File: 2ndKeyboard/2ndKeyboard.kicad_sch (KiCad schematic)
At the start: 21 parts

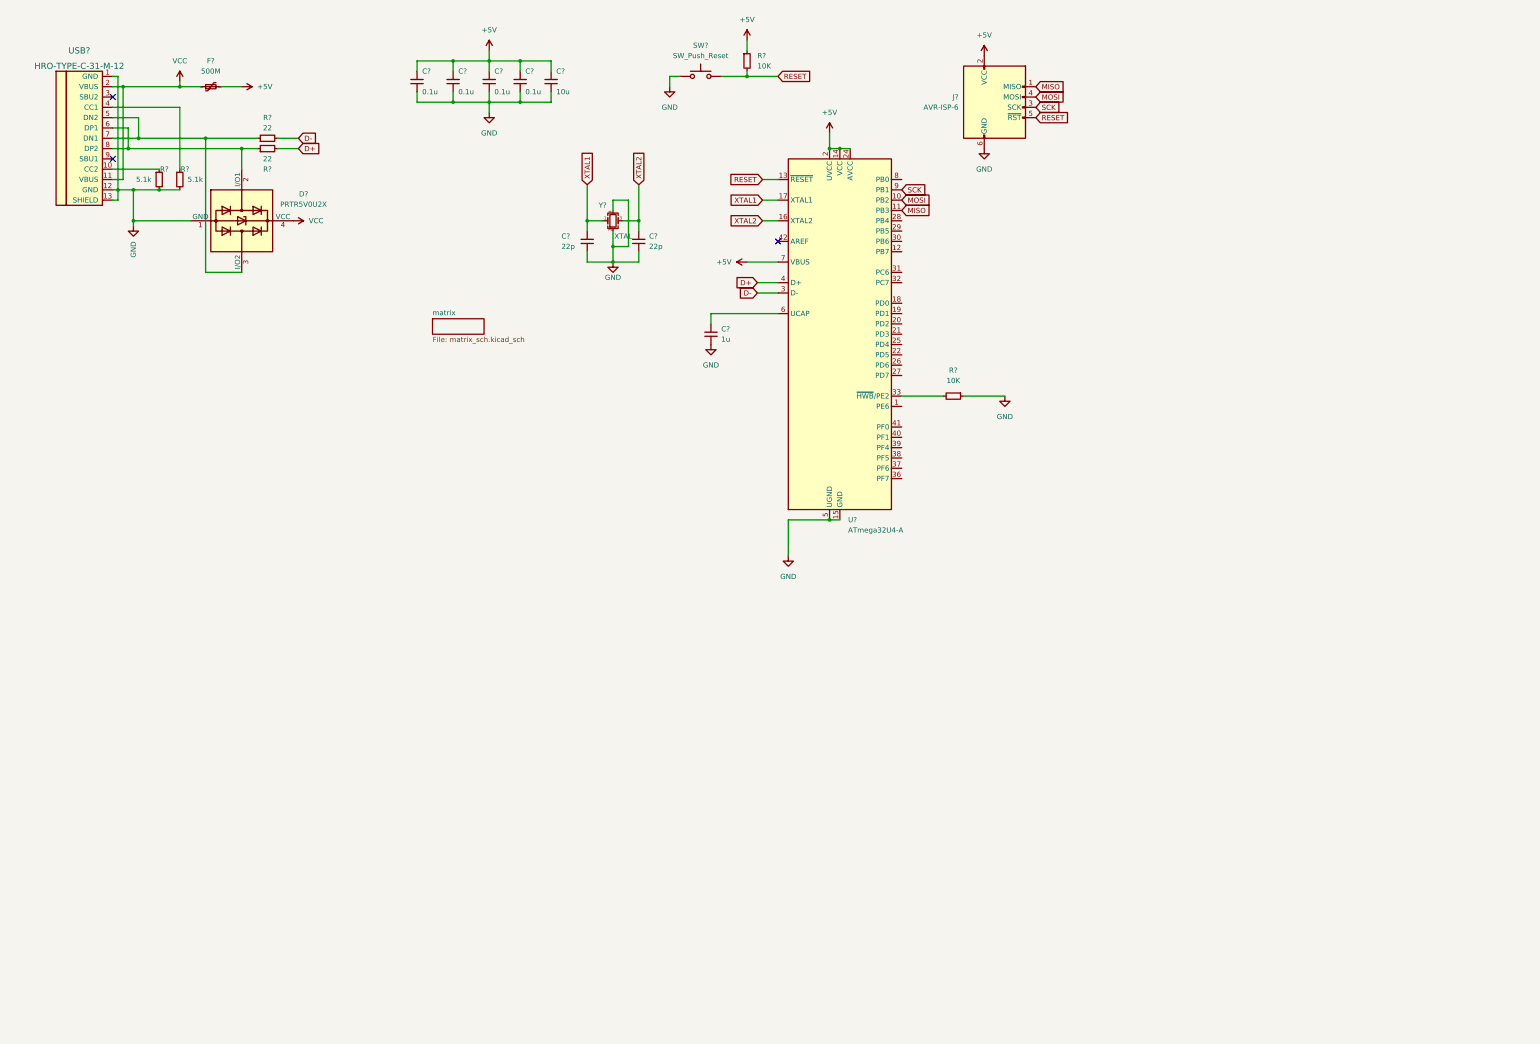
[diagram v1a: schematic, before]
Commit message: pcb
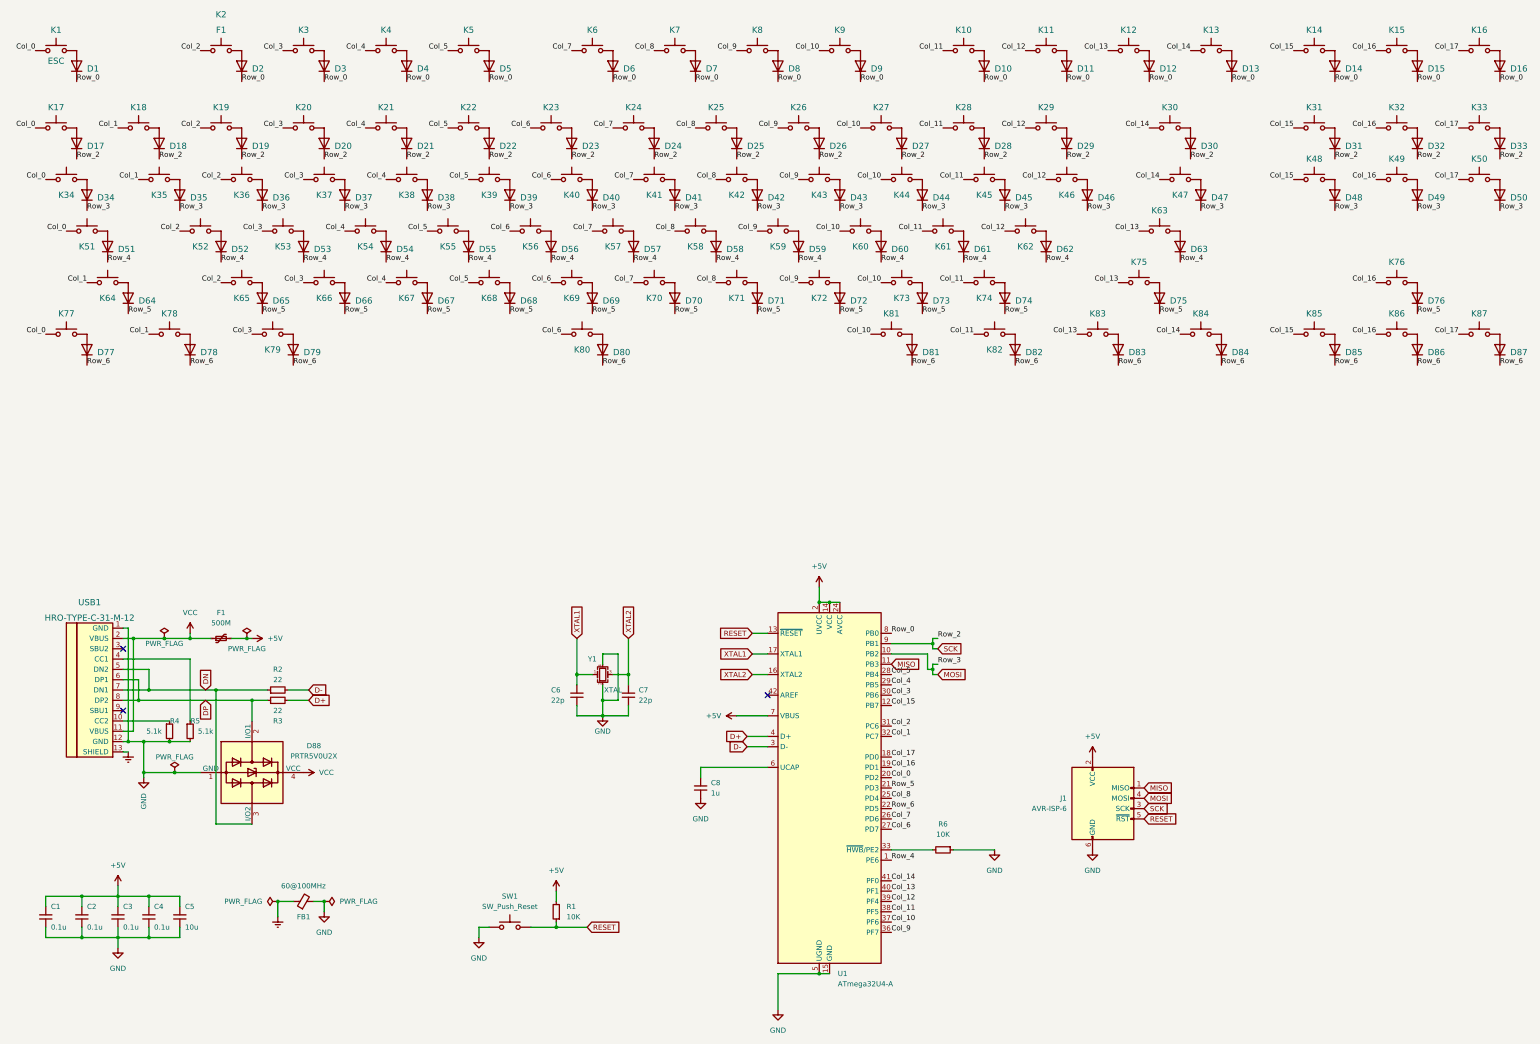
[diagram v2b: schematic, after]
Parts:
- added D1, D10, D11, D12, D13, D14, D15, D16, D17, D18, D19, D2, D20, D21, D22, D23, D24, D25, D26, D27, D28, D29, D3, D30, D31, D32, D33, D34, D35, D36, D37, D38, D39, D4, D40, D41, D42, D43, D44, D45, D46, D47, D48, D49, D5, D50, D51, D52, D53, D54, D55, D56, D57, D58, D59, D6, D60, D61, D62, D63, D64, D65, D66, D67, D68, D69, D7, D70, D71, D72, D73, D74, D75, D76, D77, D78, D79, D8, D80, D81, D82, D83, D84, D85, D86, D87, D9: D, Diode_SMD:D_SOD-123, symbol Device:D
- added FB1: 60@100MHz, Inductor_SMD:L_0805_2012Metric_Pad1.15x1.40mm_HandSolder, symbol Device:FerriteBead_Small
- added K1: ESC, Button_Switch_Keyboard:SW_Cherry_MX_1.00u_PCB, symbol Switch:SW_Push
- added K10: F9, Button_Switch_Keyboard:SW_Cherry_MX_1.00u_PCB, symbol Switch:SW_Push
- added K11: F10, Button_Switch_Keyboard:SW_Cherry_MX_1.00u_PCB, symbol Switch:SW_Push
- added K12: F11, Button_Switch_Keyboard:SW_Cherry_MX_1.00u_PCB, symbol Switch:SW_Push
- added K13: F12, Button_Switch_Keyboard:SW_Cherry_MX_1.00u_PCB, symbol Switch:SW_Push
- added K14: Imp_Ecran, Button_Switch_Keyboard:SW_Cherry_MX_1.00u_PCB, symbol Switch:SW_Push
- added K15: Defilement, Button_Switch_Keyboard:SW_Cherry_MX_1.00u_PCB, symbol Switch:SW_Push
- added K16: Pause, Button_Switch_Keyboard:SW_Cherry_MX_1.00u_PCB, symbol Switch:SW_Push
- added K17: /, Button_Switch_Keyboard:SW_Cherry_MX_1.00u_PCB, symbol Switch:SW_Push
- added K18: 1, Button_Switch_Keyboard:SW_Cherry_MX_1.00u_PCB, symbol Switch:SW_Push
- added K19: 2, Button_Switch_Keyboard:SW_Cherry_MX_1.00u_PCB, symbol Switch:SW_Push
- added K2: F1, Button_Switch_Keyboard:SW_Cherry_MX_1.00u_PCB, symbol Switch:SW_Push
- added K20: 3, Button_Switch_Keyboard:SW_Cherry_MX_1.00u_PCB, symbol Switch:SW_Push
- added K21: 4, Button_Switch_Keyboard:SW_Cherry_MX_1.00u_PCB, symbol Switch:SW_Push
- added K22: 5, Button_Switch_Keyboard:SW_Cherry_MX_1.00u_PCB, symbol Switch:SW_Push
- added K23: 6, Button_Switch_Keyboard:SW_Cherry_MX_1.00u_PCB, symbol Switch:SW_Push
- added K24: 7, Button_Switch_Keyboard:SW_Cherry_MX_1.00u_PCB, symbol Switch:SW_Push
- added K25: 8, Button_Switch_Keyboard:SW_Cherry_MX_1.00u_PCB, symbol Switch:SW_Push
- added K26: 9, Button_Switch_Keyboard:SW_Cherry_MX_1.00u_PCB, symbol Switch:SW_Push
- added K27: 0, Button_Switch_Keyboard:SW_Cherry_MX_1.00u_PCB, symbol Switch:SW_Push
- added K28: -, Button_Switch_Keyboard:SW_Cherry_MX_1.00u_PCB, symbol Switch:SW_Push
- added K29: =, Button_Switch_Keyboard:SW_Cherry_MX_1.00u_PCB, symbol Switch:SW_Push
- added K3: F2, Button_Switch_Keyboard:SW_Cherry_MX_1.00u_PCB, symbol Switch:SW_Push
- added K30: KEYSW, Button_Switch_Keyboard:SW_Cherry_MX_2.00u_PCB, symbol Switch:SW_Push
- added K31: Ins, Button_Switch_Keyboard:SW_Cherry_MX_1.00u_PCB, symbol Switch:SW_Push
- added K32: Debut, Button_Switch_Keyboard:SW_Cherry_MX_1.00u_PCB, symbol Switch:SW_Push
- added K33: Next, Button_Switch_Keyboard:SW_Cherry_MX_1.00u_PCB, symbol Switch:SW_Push
- added K34: TAB, Button_Switch_Keyboard:SW_Cherry_MX_1.25u_PCB, symbol Switch:SW_Push
- added K35: Q, Button_Switch_Keyboard:SW_Cherry_MX_1.00u_PCB, symbol Switch:SW_Push
- added K36: W, Button_Switch_Keyboard:SW_Cherry_MX_1.00u_PCB, symbol Switch:SW_Push
- added K37: E, Button_Switch_Keyboard:SW_Cherry_MX_1.00u_PCB, symbol Switch:SW_Push
- added K38: R, Button_Switch_Keyboard:SW_Cherry_MX_1.00u_PCB, symbol Switch:SW_Push
- added K39: T, Button_Switch_Keyboard:SW_Cherry_MX_1.00u_PCB, symbol Switch:SW_Push
- added K4: F3, Button_Switch_Keyboard:SW_Cherry_MX_1.00u_PCB, symbol Switch:SW_Push
- added K40: Y, Button_Switch_Keyboard:SW_Cherry_MX_1.00u_PCB, symbol Switch:SW_Push
- added K41: U, Button_Switch_Keyboard:SW_Cherry_MX_1.00u_PCB, symbol Switch:SW_Push
- added K42: I, Button_Switch_Keyboard:SW_Cherry_MX_1.00u_PCB, symbol Switch:SW_Push
- added K43: O, Button_Switch_Keyboard:SW_Cherry_MX_1.00u_PCB, symbol Switch:SW_Push
- added K44: P, Button_Switch_Keyboard:SW_Cherry_MX_1.00u_PCB, symbol Switch:SW_Push
- added K45: ^, Button_Switch_Keyboard:SW_Cherry_MX_1.00u_PCB, symbol Switch:SW_Push
- added K46: Ç, Button_Switch_Keyboard:SW_Cherry_MX_1.00u_PCB, symbol Switch:SW_Push
- added K47: À, Button_Switch_Keyboard:SW_Cherry_MX_1.75u_PCB, symbol Switch:SW_Push
- added K48: Suppr, Button_Switch_Keyboard:SW_Cherry_MX_1.00u_PCB, symbol Switch:SW_Push
- added K49: FIN, Button_Switch_Keyboard:SW_Cherry_MX_1.00u_PCB, symbol Switch:SW_Push
- added K5: F4, Button_Switch_Keyboard:SW_Cherry_MX_1.00u_PCB, symbol Switch:SW_Push
- added K50: Previous, Button_Switch_Keyboard:SW_Cherry_MX_1.00u_PCB, symbol Switch:SW_Push
- added K51: CAPS LOCK, Button_Switch_Keyboard:SW_Cherry_MX_1.75u_PCB, symbol Switch:SW_Push
- added K52: A, Button_Switch_Keyboard:SW_Cherry_MX_1.00u_PCB, symbol Switch:SW_Push
- added K53: S, Button_Switch_Keyboard:SW_Cherry_MX_1.00u_PCB, symbol Switch:SW_Push
- added K54: D, Button_Switch_Keyboard:SW_Cherry_MX_1.00u_PCB, symbol Switch:SW_Push
- added K55: F, Button_Switch_Keyboard:SW_Cherry_MX_1.00u_PCB, symbol Switch:SW_Push
- added K56: G, Button_Switch_Keyboard:SW_Cherry_MX_1.00u_PCB, symbol Switch:SW_Push
- added K57: H, Button_Switch_Keyboard:SW_Cherry_MX_1.00u_PCB, symbol Switch:SW_Push
- added K58: J, Button_Switch_Keyboard:SW_Cherry_MX_1.00u_PCB, symbol Switch:SW_Push
- added K59: K, Button_Switch_Keyboard:SW_Cherry_MX_1.00u_PCB, symbol Switch:SW_Push
- added K6: F5, Button_Switch_Keyboard:SW_Cherry_MX_1.00u_PCB, symbol Switch:SW_Push
- added K60: L, Button_Switch_Keyboard:SW_Cherry_MX_1.00u_PCB, symbol Switch:SW_Push
- added K61: ;, Button_Switch_Keyboard:SW_Cherry_MX_1.00u_PCB, symbol Switch:SW_Push
- added K62: È, Button_Switch_Keyboard:SW_Cherry_MX_1.00u_PCB, symbol Switch:SW_Push
- added K63: ENTER, Button_Switch_Keyboard:SW_Cherry_MX_2.25u_PCB, symbol Switch:SW_Push
- added K64: MAJ G., Button_Switch_Keyboard:SW_Cherry_MX_2.25u_PCB, symbol Switch:SW_Push
- added K65: Z, Button_Switch_Keyboard:SW_Cherry_MX_1.00u_PCB, symbol Switch:SW_Push
- added K66: X, Button_Switch_Keyboard:SW_Cherry_MX_1.00u_PCB, symbol Switch:SW_Push
- added K67: C, Button_Switch_Keyboard:SW_Cherry_MX_1.00u_PCB, symbol Switch:SW_Push
- added K68: V, Button_Switch_Keyboard:SW_Cherry_MX_1.00u_PCB, symbol Switch:SW_Push
- added K69: B, Button_Switch_Keyboard:SW_Cherry_MX_1.00u_PCB, symbol Switch:SW_Push
- added K7: F6, Button_Switch_Keyboard:SW_Cherry_MX_1.00u_PCB, symbol Switch:SW_Push
- added K70: N, Button_Switch_Keyboard:SW_Cherry_MX_1.00u_PCB, symbol Switch:SW_Push
- added K71: M, Button_Switch_Keyboard:SW_Cherry_MX_1.00u_PCB, symbol Switch:SW_Push
- added K72: ,, Button_Switch_Keyboard:SW_Cherry_MX_1.00u_PCB, symbol Switch:SW_Push
- added K73: ., Button_Switch_Keyboard:SW_Cherry_MX_1.00u_PCB, symbol Switch:SW_Push
- added K74: É, Button_Switch_Keyboard:SW_Cherry_MX_1.00u_PCB, symbol Switch:SW_Push
- added K75: MAJ D., Button_Switch_Keyboard:SW_Cherry_MX_2.75u_PCB, symbol Switch:SW_Push
- added K76: UP Arrow, Button_Switch_Keyboard:SW_Cherry_MX_1.00u_PCB, symbol Switch:SW_Push
- added K77: CTRL G., Button_Switch_Keyboard:SW_Cherry_MX_1.25u_PCB, symbol Switch:SW_Push
- added K78, K82: WINDOWS, Button_Switch_Keyboard:SW_Cherry_MX_1.25u_PCB, symbol Switch:SW_Push
- added K79: ALT G., Button_Switch_Keyboard:SW_Cherry_MX_1.25u_PCB, symbol Switch:SW_Push
- added K8: F7, Button_Switch_Keyboard:SW_Cherry_MX_1.00u_PCB, symbol Switch:SW_Push
- added K80: BARRE, Button_Switch_Keyboard:SW_Cherry_MX_6.25u_PCB, symbol Switch:SW_Push
- added K81: ALT D., Button_Switch_Keyboard:SW_Cherry_MX_1.25u_PCB, symbol Switch:SW_Push
- added K83: MENU, Button_Switch_Keyboard:SW_Cherry_MX_1.25u_PCB, symbol Switch:SW_Push
- added K84: CTRL D., Button_Switch_Keyboard:SW_Cherry_MX_1.25u_PCB, symbol Switch:SW_Push
- added K85: LEFT Arrow, Button_Switch_Keyboard:SW_Cherry_MX_1.00u_PCB, symbol Switch:SW_Push
- added K86: DOWN Arrow, Button_Switch_Keyboard:SW_Cherry_MX_1.00u_PCB, symbol Switch:SW_Push
- added K87: RIGHT Arrow, Button_Switch_Keyboard:SW_Cherry_MX_1.00u_PCB, symbol Switch:SW_Push
- added K9: F8, Button_Switch_Keyboard:SW_Cherry_MX_1.00u_PCB, symbol Switch:SW_Push
- C1, C2, C3, C4, C5, C6, C7, C8: renamed from C?; footprint (none) -> Capacitor_SMD:C_0805_2012Metric_Pad1.18x1.45mm_HandSolder
- D88: renamed from D?; footprint Package_TO_SOT_SMD:SOT-143 -> random-keyboard-parts:SOT143B
- F1: renamed from F?; footprint (none) -> Fuse:Fuse_1206_3216Metric_Pad1.42x1.75mm_HandSolder
- J1: renamed from J?; footprint (none) -> random-keyboard-parts:Reset_Pretty-Mask
- R1, R2, R3, R4, R5, R6: renamed from R?; footprint (none) -> Resistor_SMD:R_0805_2012Metric_Pad1.20x1.40mm_HandSolder
- SW1: renamed from SW?; footprint (none) -> Button_Switch_SMD:SW_SPST_SKQG_WithStem
- USB1: renamed from USB?; footprint (none) -> Type-C:HRO-TYPE-C-31-M-12-HandSoldering
- Y1: renamed from Y?; footprint (none) -> Crystal:Crystal_SMD_3225-4Pin_3.2x2.5mm_HandSoldering
- gave numbers to parts that had none: 1
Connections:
- net +5V: now also R1.2; no longer R1.1
- net GND: now also FB1.2; no longer USB1.13 (SHIELD)
- net MOSI: now also D34.1 (K), D35.1 (K), D36.1 (K), D37.1 (K), D38.1 (K), D39.1 (K), D40.1 (K), D41.1 (K), D42.1 (K), D43.1 (K), D44.1 (K), D45.1 (K), D46.1 (K), D47.1 (K), D48.1 (K), D49.1 (K), D50.1 (K)
- net RESET: now also R1.1; no longer R1.2
- net SCK: now also D17.1 (K), D18.1 (K), D19.1 (K), D20.1 (K), D21.1 (K), D22.1 (K), D23.1 (K), D24.1 (K), D25.1 (K), D26.1 (K), D27.1 (K), D28.1 (K), D29.1 (K), D30.1 (K), D31.1 (K), D32.1 (K), D33.1 (K)
- net DN: now reaches D88.3 (I/O2), R2.1, USB1.5 (DN2), USB1.7 (DN1)
- net DP: now reaches D88.2 (I/O1), R3.1, USB1.6 (DP1), USB1.8 (DP2)
- net Row_4: now reaches U1.1 (PE6)
- net Row_4: now also D51.1 (K), D52.1 (K), D53.1 (K), D54.1 (K), D55.1 (K), D56.1 (K), D57.1 (K), D58.1 (K), D59.1 (K), D60.1 (K), D61.1 (K), D62.1 (K), D63.1 (K)
- net Col_15: now reaches U1.12 (PB7)
- net Col_15: now also K14.1, K31.1, K48.1, K85.1
- net Col_17: now reaches U1.18 (PD0)
- net Col_17: now also K16.1, K33.1, K50.1, K87.1
- net Col_16: now reaches U1.19 (PD1)
- net Col_16: now also K15.1, K32.1, K49.1, K76.1, K86.1
- net Col_0: now reaches U1.20 (PD2)
- net Col_0: now also K1.1, K17.1, K34.1, K51.1, K77.1
- net Row_5: now reaches U1.21 (PD3)
- net Row_5: now also D64.1 (K), D65.1 (K), D66.1 (K), D67.1 (K), D68.1 (K), D69.1 (K), D70.1 (K), D71.1 (K), D72.1 (K), D73.1 (K), D74.1 (K), D75.1 (K), D76.1 (K)
- net Row_6: now reaches U1.22 (PD5)
- net Row_6: now also D77.1 (K), D78.1 (K), D79.1 (K), D80.1 (K), D81.1 (K), D82.1 (K), D83.1 (K), D84.1 (K), D85.1 (K), D86.1 (K), D87.1 (K)
- net Col_8: now reaches U1.25 (PD4)
- net Col_8: now also K25.1, K42.1, K58.1, K7.1, K71.1
- net Col_7: now reaches U1.26 (PD6)
- net Col_7: now also K24.1, K41.1, K57.1, K6.1, K70.1
- net Col_6: now reaches U1.27 (PD7)
- net Col_6: now also K23.1, K40.1, K56.1, K69.1, K80.1
- net Col_5: now reaches U1.28 (PB4)
- net Col_5: now also K22.1, K39.1, K5.1, K55.1, K68.1
- net Col_4: now reaches U1.29 (PB5)
- net Col_4: now also K21.1, K38.1, K4.1, K54.1, K67.1
- net Col_3: now reaches U1.30 (PB6)
- net Col_3: now also K20.1, K3.1, K37.1, K53.1, K66.1, K79.1
- net Col_2: now reaches U1.31 (PC6)
- net Col_2: now also K19.1, K2.1, K36.1, K52.1, K65.1
- net Col_1: now reaches U1.32 (PC7)
- net Col_1: now also K18.1, K35.1, K64.1, K78.1
- net Col_9: now reaches U1.36 (PF7)
- net Col_9: now also K26.1, K43.1, K59.1, K72.1, K8.1
- net Col_10: now reaches U1.37 (PF6)
- net Col_10: now also K27.1, K44.1, K60.1, K73.1, K81.1, K9.1
- net Col_11: now reaches U1.38 (PF5)
- net Col_11: now also K10.1, K28.1, K45.1, K61.1, K74.1, K82.1
- net Col_12: now reaches U1.39 (PF4)
- net Col_12: now also K11.1, K29.1, K46.1, K62.1
- net Col_13: now reaches U1.40 (PF1)
- net Col_13: now also K12.1, K63.1, K75.1, K83.1
- net Col_14: now reaches U1.41 (PF0)
- net Col_14: now also K13.1, K30.1, K47.1, K84.1
- net Row_0: now reaches U1.8 (PB0)
- net Row_0: now also D1.1 (K), D10.1 (K), D11.1 (K), D12.1 (K), D13.1 (K), D14.1 (K), D15.1 (K), D16.1 (K), D2.1 (K), D3.1 (K), D4.1 (K), D5.1 (K), D6.1 (K), D7.1 (K), D8.1 (K), D9.1 (K)
- new net: D62.2 (A), K62.2
- new net: D66.2 (A), K66.2
- new net: D50.2 (A), K50.2
- new net: D12.2 (A), K12.2
- new net: D40.2 (A), K40.2
- new net: D58.2 (A), K58.2
- new net: D59.2 (A), K59.2
- new net: D75.2 (A), K75.2
- new net: D32.2 (A), K32.2
- new net: D73.2 (A), K73.2
- new net: D23.2 (A), K23.2
- new net: D56.2 (A), K56.2
- new net: D1.2 (A), K1.2
- new net: D30.2 (A), K30.2
- new net: D83.2 (A), K83.2
- new net: D79.2 (A), K79.2
- new net: D64.2 (A), K64.2
- new net: D43.2 (A), K43.2
- new net: D57.2 (A), K57.2
- new net: D72.2 (A), K72.2
- new net: D17.2 (A), K17.2
- new net: D80.2 (A), K80.2
- new net: D44.2 (A), K44.2
- new net: D60.2 (A), K60.2
- new net: D48.2 (A), K48.2
- new net: D7.2 (A), K7.2
- new net: D41.2 (A), K41.2
- new net: D67.2 (A), K67.2
- new net: D13.2 (A), K13.2
- new net: D31.2 (A), K31.2
- new net: D4.2 (A), K4.2
- new net: D19.2 (A), K19.2
- new net: D42.2 (A), K42.2
- new net: D37.2 (A), K37.2
- new net: D65.2 (A), K65.2
- new net: D16.2 (A), K16.2
- new net: D53.2 (A), K53.2
- new net: D69.2 (A), K69.2
- new net: D86.2 (A), K86.2
- new net: D76.2 (A), K76.2
- new net: D20.2 (A), K20.2
- new net: D2.2 (A), K2.2
- new net: D54.2 (A), K54.2
- new net: D34.2 (A), K34.2
- new net: D70.2 (A), K70.2
- new net: D14.2 (A), K14.2
- new net: D71.2 (A), K71.2
- new net: D9.2 (A), K9.2
- new net: D38.2 (A), K38.2
- new net: D45.2 (A), K45.2
- new net: D68.2 (A), K68.2
- new net: D49.2 (A), K49.2
- new net: D11.2 (A), K11.2
- new net: D10.2 (A), K10.2
- new net: D35.2 (A), K35.2
- new net: D33.2 (A), K33.2
- new net: D3.2 (A), K3.2
- new net: D25.2 (A), K25.2
- new net: D27.2 (A), K27.2
- new net: D5.2 (A), K5.2
- new net: D46.2 (A), K46.2
- new net: D39.2 (A), K39.2
- new net: D26.2 (A), K26.2
- new net: D47.2 (A), K47.2
- new net: D36.2 (A), K36.2
- new net: D78.2 (A), K78.2
- new net: D81.2 (A), K81.2
- new net: D82.2 (A), K82.2
- new net: D22.2 (A), K22.2
- new net: D28.2 (A), K28.2
- new net: D63.2 (A), K63.2
- new net: D15.2 (A), K15.2
- new net: D8.2 (A), K8.2
- new net: D6.2 (A), K6.2
- new net: D61.2 (A), K61.2
- new net: D24.2 (A), K24.2
- new net: D74.2 (A), K74.2
- new net: D84.2 (A), K84.2
- new net: D21.2 (A), K21.2
- new net: D87.2 (A), K87.2
- new net: D77.2 (A), K77.2
- new net: D29.2 (A), K29.2
- new net: D52.2 (A), K52.2
- new net: D51.2 (A), K51.2
- new net: D18.2 (A), K18.2
- new net: D85.2 (A), K85.2
- new net: D55.2 (A), K55.2
- new net Earth: FB1.1, USB1.13 (SHIELD)
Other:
- removed sheet matrix
- moved on the sheet: C1, C2, C3, C4, C5, C6, C7, C8, D88, F1, J1, R1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

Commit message: pcb3
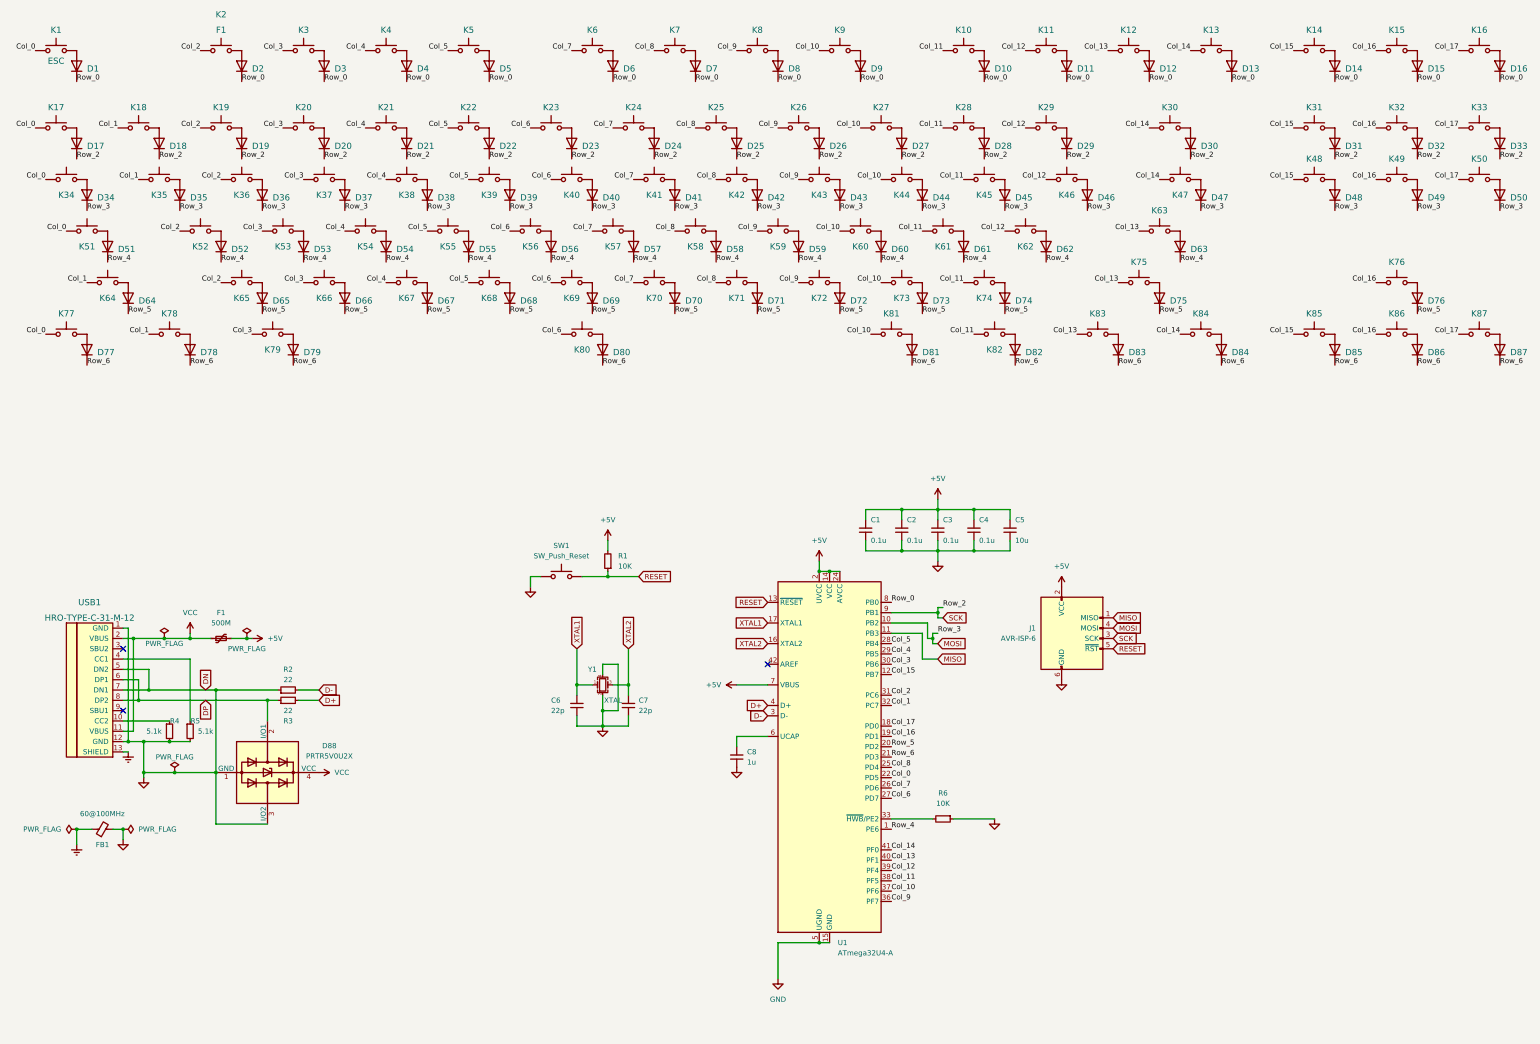
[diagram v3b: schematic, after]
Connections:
- net DN is gone; now on net GND: D88.3 (I/O2), R2.1, USB1.5 (DN2), USB1.7 (DN1)
- net Col_0: now also U1.22 (PD5); no longer U1.20 (PD2)
- net Row_5: now also U1.20 (PD2); no longer U1.21 (PD3)
- net Row_6: now also U1.21 (PD3); no longer U1.22 (PD5)
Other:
- moved on the sheet: C1, C2, C3, C4, C5, C6, C7, C8, D88, FB1, J1, R1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

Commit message: pcb reviewed 07-01-23
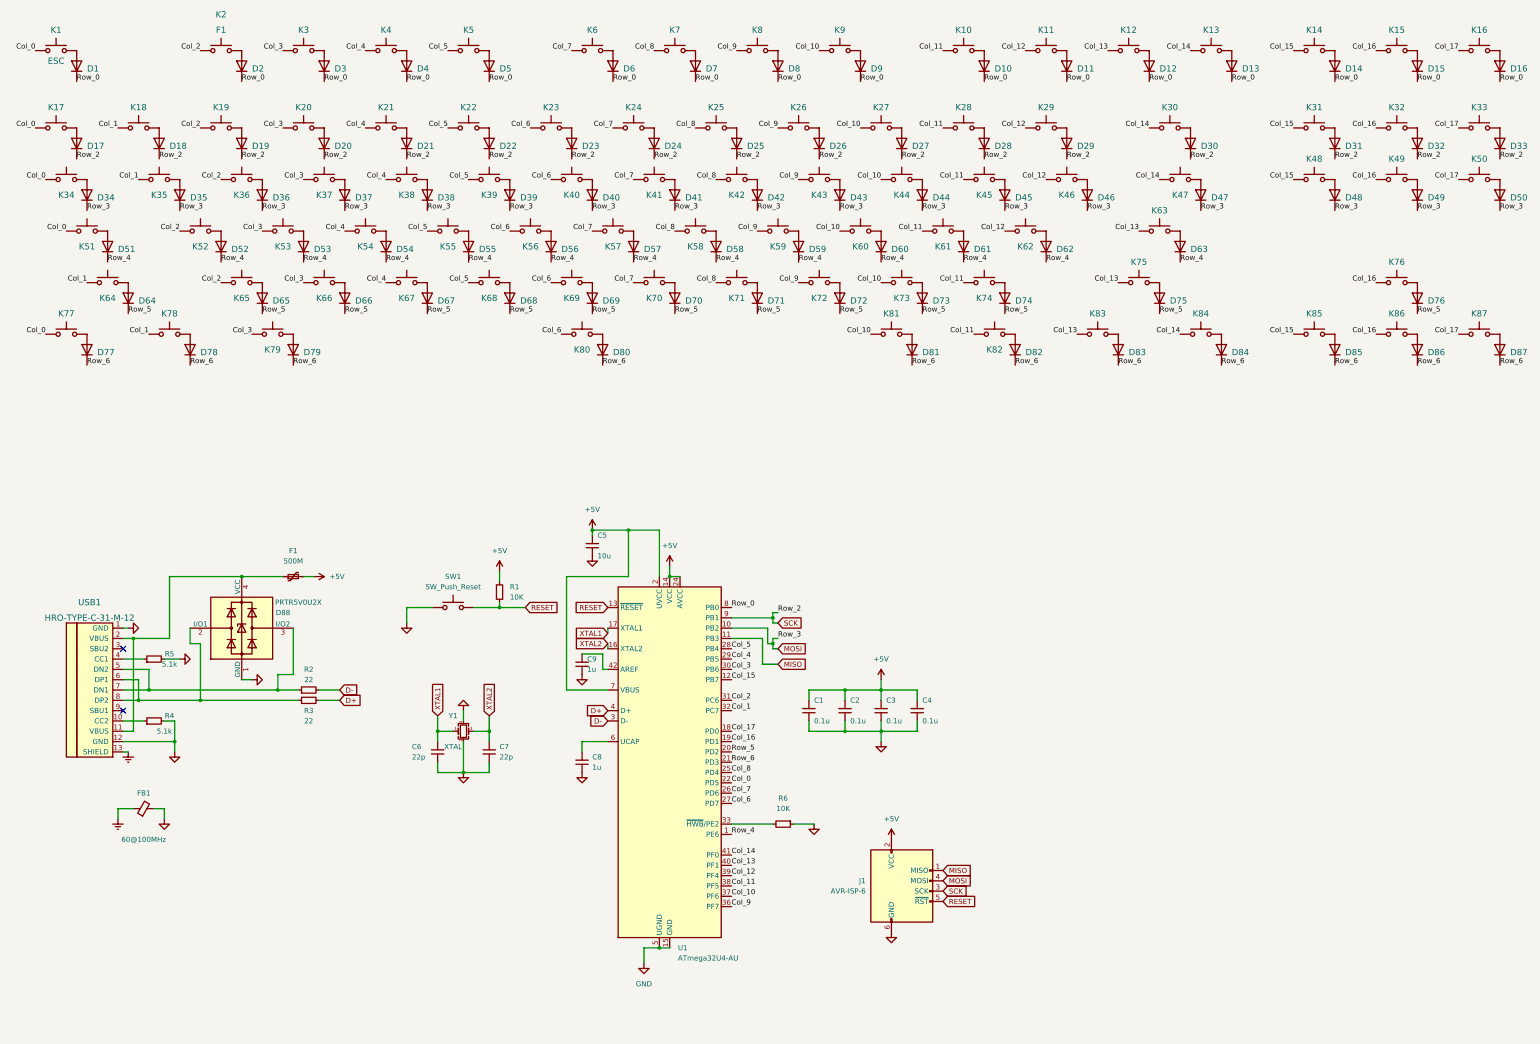
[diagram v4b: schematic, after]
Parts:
- added C9: 1u, Capacitor_SMD:C_0805_2012Metric_Pad1.18x1.45mm_HandSolder, symbol Device:C_Small
- U1: value ATmega32U4-A -> ATmega32U4-AU
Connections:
- net GND: now also C9.1; no longer D88.3 (I/O2), R2.1, USB1.5 (DN2), USB1.7 (DN1)
- net at U1.42 (AREF): now also C9.2
- net DP: no longer names the net of D88.2 (I/O1), R3.1, USB1.6 (DP1), USB1.8 (DP2)
- net VCC: no longer names the net of D88.4 (VCC), F1.1, USB1.11 (VBUS), USB1.2 (VBUS)
- new net: D88.3 (I/O2), R2.1, USB1.5 (DN2), USB1.7 (DN1)
- no-connect marks 3 -> 2
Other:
- moved on the sheet: C1, C2, C3, C4, C5, C6, C7, C8, D88, F1, FB1, J1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
